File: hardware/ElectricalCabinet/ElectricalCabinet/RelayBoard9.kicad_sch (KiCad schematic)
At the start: 0 parts

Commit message: Further wiring updates
Populated 6100 Bus
Corrected number of relay boards
Added 110v outputs to relay boards and noted light positon
Uploaded light scheme to documents folder
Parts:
- added C9: 0.1uF, Capacitor_SMD:C_0805_2012Metric, symbol Device:C
- added D65, D66, D67, D68, D69, D70, D71, D72: LED, LED_SMD:LED_0805_2012Metric, symbol Device:LED
- added J18: Screw_Terminal_01x06, TerminalBlock:TerminalBlock_MaiXu_MX126-5.0-06P_1x06_P5.00mm, symbol Connector:Screw_Terminal_01x06
- added J19: Screw_Terminal_01x09, TerminalBlock:TerminalBlock_MaiXu_MX126-5.0-09P_1x09_P5.00mm, symbol Connector:Screw_Terminal_01x09
- added K65, K66, K67, K68, K69, K70, K71, K72: G3MB-202P DC5, TrafficLightLibrary:G3MB_202P_DC5, symbol TrafficLightLibrary:G3MB-202P_DC5
- added R65, R66, R67, R68, R69, R70, R71, R72: 1kΩ, Resistor_SMD:R_0805_2012Metric, symbol Device:R
- added U10: TPIC6B595N, TrafficLightLibrary:TPIC6B595N, symbol TrafficLightLibrary:TPIC6B595N
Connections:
- new net: D66.1 (K), R66.1
- new net: D65.2 (A), D66.2 (A), D67.2 (A), D68.2 (A), D69.2 (A), D70.2 (A), D71.2 (A), D72.2 (A), K65.3, K66.3, K67.3, K68.3, K69.3, K70.3, K71.3, K72.3
- new net: D70.1 (K), R70.1
- new net: K70.4, R70.2, U10.15 (DRAIN5)
- new net: J19.1 (Pin_1), K65.2
- new net: J19.2 (Pin_2), K66.2
- new net: J19.3 (Pin_3), K67.2
- new net: J19.4 (Pin_4), K68.2
- new net: J19.5 (Pin_5), K69.2
- new net: J19.6 (Pin_6), K70.2
- new net: J19.7 (Pin_7), K71.2
- new net: J19.8 (Pin_8), K72.2
- new net: J19.9 (Pin_9), K65.1, K66.1, K67.1, K68.1, K69.1, K70.1, K71.1, K72.1
- new net: D72.1 (K), R72.1
- new net: K68.4, R68.2, U10.7 (DRAIN3)
- new net: D65.1 (K), R65.1
- new net: D71.1 (K), R71.1
- new net: K66.4, R66.2, U10.5 (DRAIN1)
- new net: D68.1 (K), R68.1
- new net: K67.4, R67.2, U10.6 (DRAIN2)
- new net: K65.4, R65.2, U10.4 (DRAIN0)
- new net: D67.1 (K), R67.1
- new net: K72.4, R72.2, U10.17 (DRAIN7)
- new net: K71.4, R71.2, U10.16 (DRAIN6)
- new net: D69.1 (K), R69.1
- new net: K69.4, R69.2, U10.14 (DRAIN4)
- new net: C9.1, J18.2 (Pin_2), U10.10 (GND), U10.11 (GND), U10.19 (GND), U10.9 (~{G})
- new net: C9.2, J18.6 (Pin_6), U10.2 (VCC), U10.8 (~{SRCLR})
- new net: J18.1 (Pin_1), U10.18 (SEROUT)
- new net: J18.3 (Pin_3), U10.13 (SRCK)
- new net: J18.4 (Pin_4), U10.12 (RCK)
- new net SERIN: J18.5 (Pin_5), U10.3 (SERIN)
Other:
- note added: "RELAY MODULE 9"

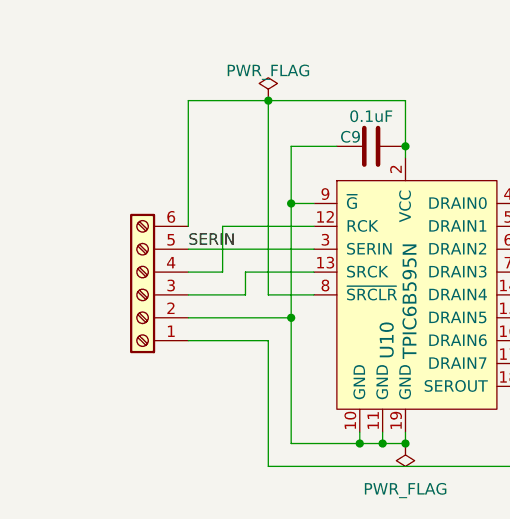
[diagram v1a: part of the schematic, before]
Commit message: Electrical Cabinet done
Electrical Cabinet done, let me know if there are any changes or mistakes.
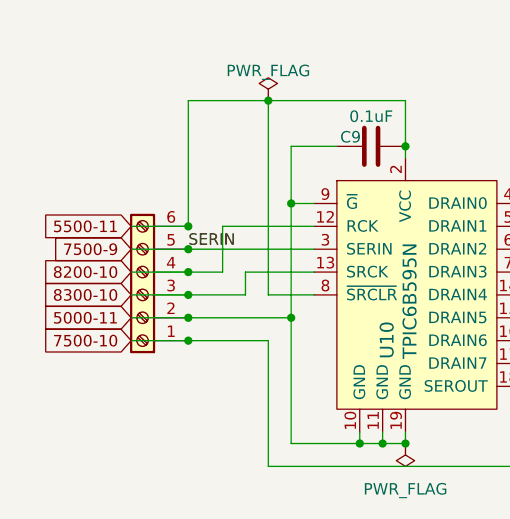
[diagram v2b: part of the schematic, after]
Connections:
- net 5000-11: now reaches C9.1, J18.2 (Pin_2), U10.10 (GND), U10.11 (GND), U10.19 (GND), U10.9 (~{G})
- net 5500-11: now reaches C9.2, J18.6 (Pin_6), U10.2 (VCC), U10.8 (~{SRCLR})
- net 7500-10: now reaches J18.1 (Pin_1), U10.18 (SEROUT)
- net 8300-10: now reaches J18.3 (Pin_3), U10.13 (SRCK)
- net 8200-10: now reaches J18.4 (Pin_4), U10.12 (RCK)
- net SERIN renamed 7500-9
